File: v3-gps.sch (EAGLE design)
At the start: 182 parts, among them IC1 XC2C32A_VQ44_2, J1 1.27MM-SWD-CONNECTOR, J2 CON_SMA-ENDFIRE_EMERSON_EMERS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, J3 ROCKETNET-CONNECTOR-16M, J4 ZX62D-B-5P8, J7 CON_HIROSE_DM3D(MICROSD), Q1 NTR4101P, T1 ALT4532, T2 ALT4532, U1 MAX2769, U10 BP2G+, U11 MAX8510EXK29+T, U12 AVAGO-ALM-GPXX, U2 STM32F4V_100PIN_GPSBOARD, U3 KSZ8081, U4 7Q-16.368MBG-T, U6 MAX8510EXK29+T, U7 MAX8510EXK29+T, U8 LMZ12001, U9 VENUS638FLPX-L, X1 25 MHz

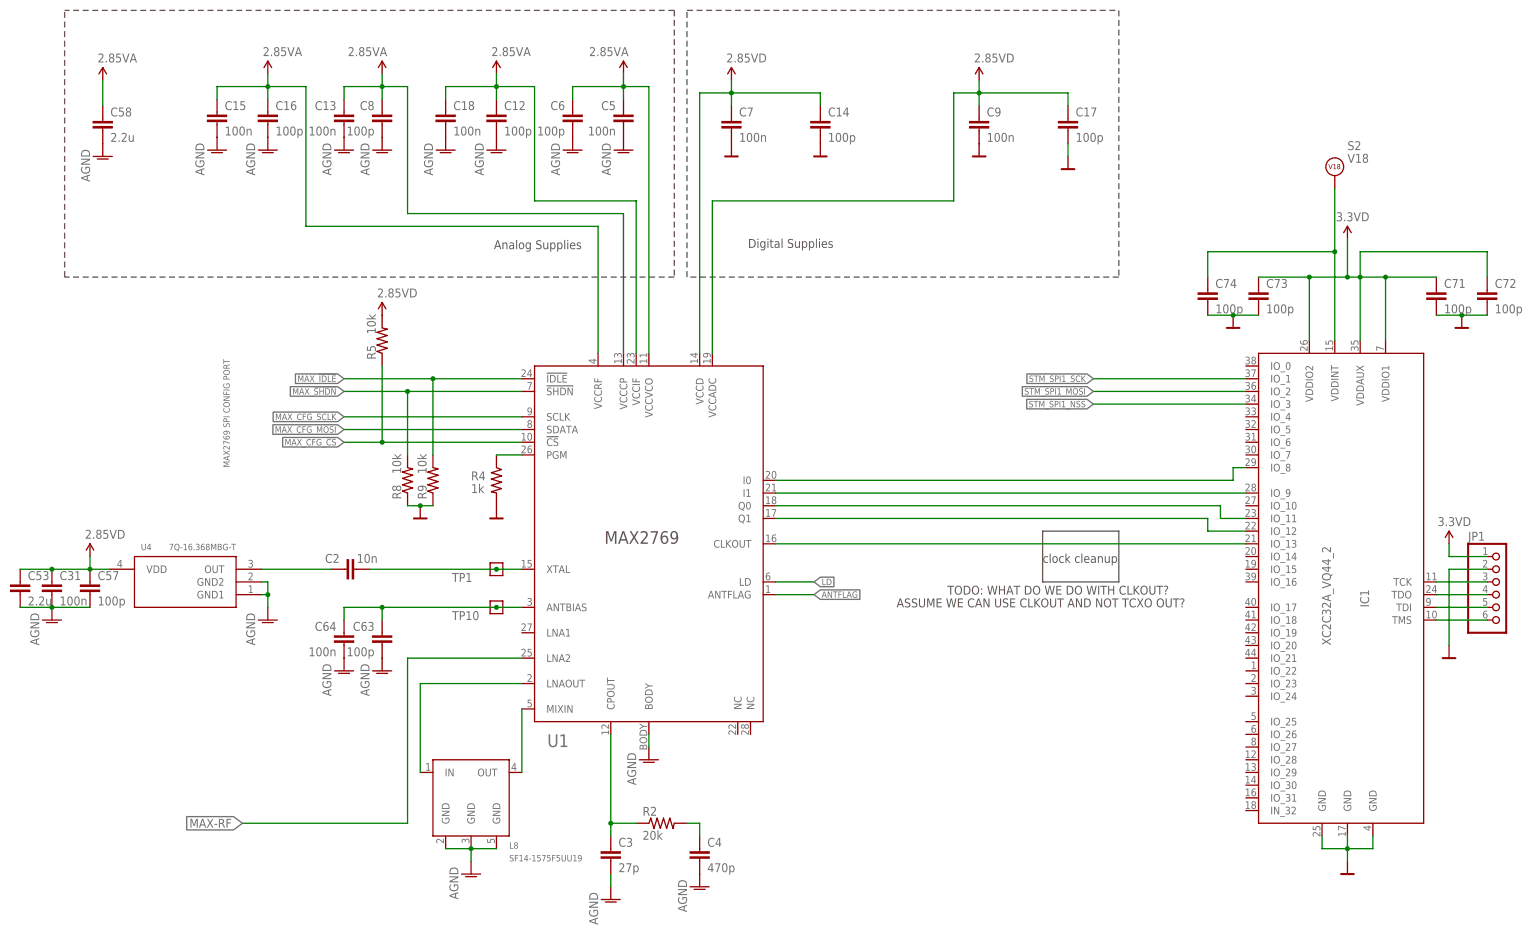
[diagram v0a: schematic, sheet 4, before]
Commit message: Couldn't help myself; wired all the things. Left to do: clean-up, mostly. Verify CPLD pins, verify MAX connections and SkyTraq connections, design review, etc.
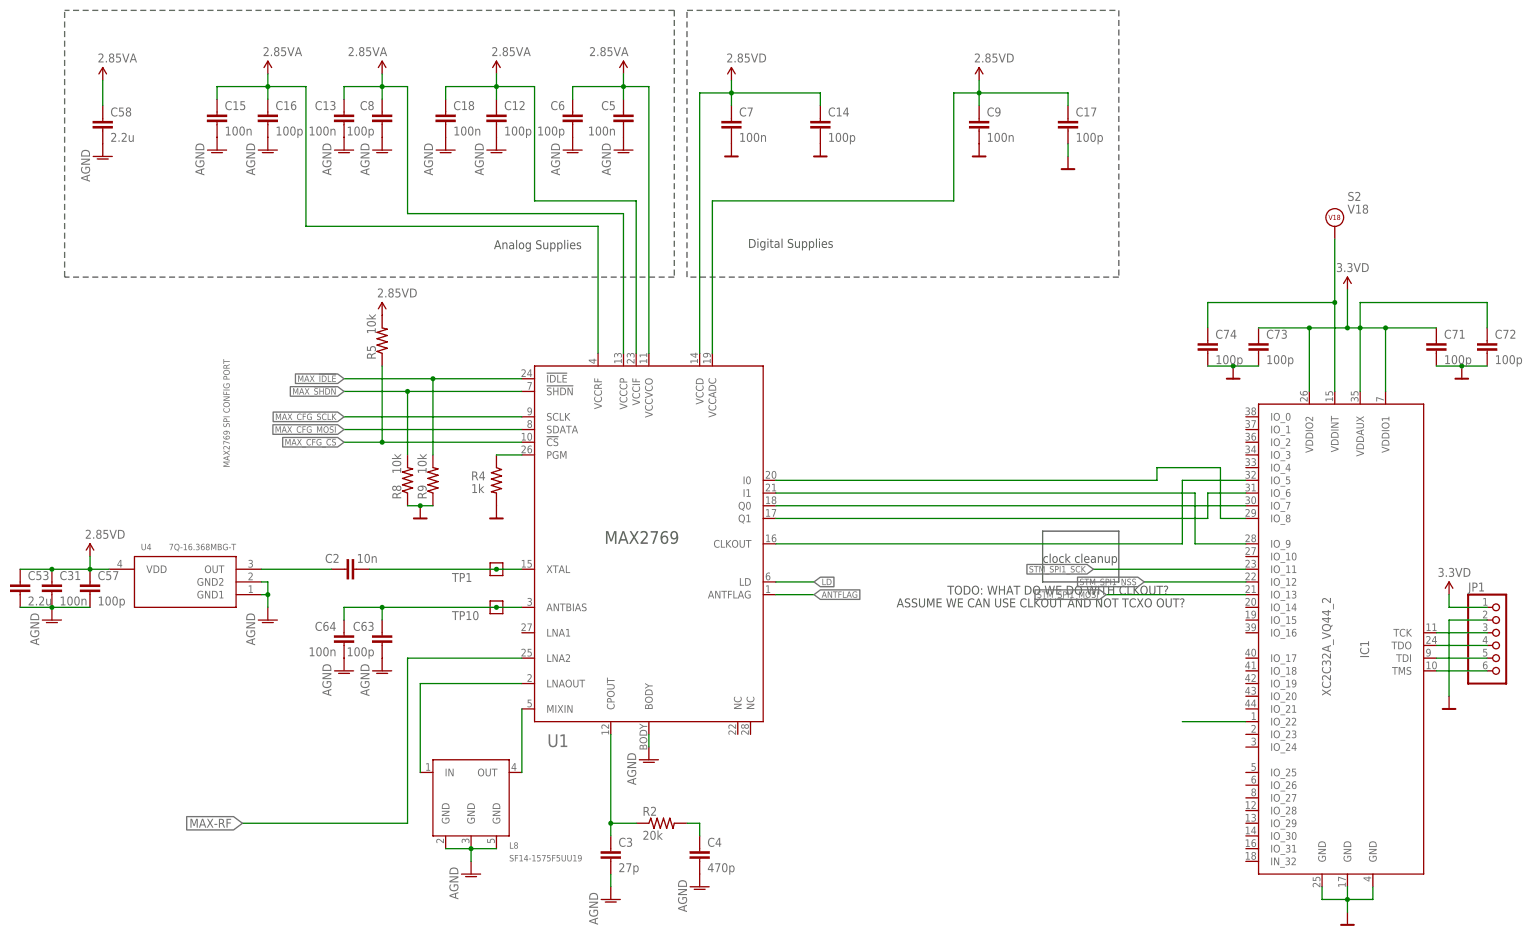
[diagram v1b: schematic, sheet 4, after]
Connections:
- net N$43 renamed VCAP_1
- net N$45 renamed VCAP_2
- net N$9 renamed BOOT0
- new net N$9: IC1.IO_22
- net N$64: now also IC1.IO_5; no longer IC1.IO_13
- net Q0: now also IC1.IO_7; no longer IC1.IO_11
- net Q1: now also IC1.IO_6; no longer IC1.IO_12
- net STM_SPI1_MOSI: now also IC1.IO_13; no longer IC1.IO_2
- net STM_SPI1_NSS: now also IC1.IO_12; no longer IC1.IO_3
- net STM_SPI1_SCK: now also IC1.IO_11; no longer IC1.IO_1
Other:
- moved on the sheet: C71, C72, C73, C74, IC1, JP1
